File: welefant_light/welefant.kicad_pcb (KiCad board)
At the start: 2 copper layers, 80 x 90 mm, 97 parts, among them J1 Conn_01x02, J2 Conn_02x8_Odd_Even, J3 Conn_02x6_Odd_Even, Q1 AO3401A, Q2 AO3401A, Q3 AO3401A, SW1 DPDT, SW2 RESET, SW3 BOOT, U1 NCP167BMX330TBG, U2 Audio Jack PJ-324, U3 SD18OB261-060, U4 TP4056, U5 welefant, U7 ESP32-S3, U8 128MBit Flash, X1 40 MHz

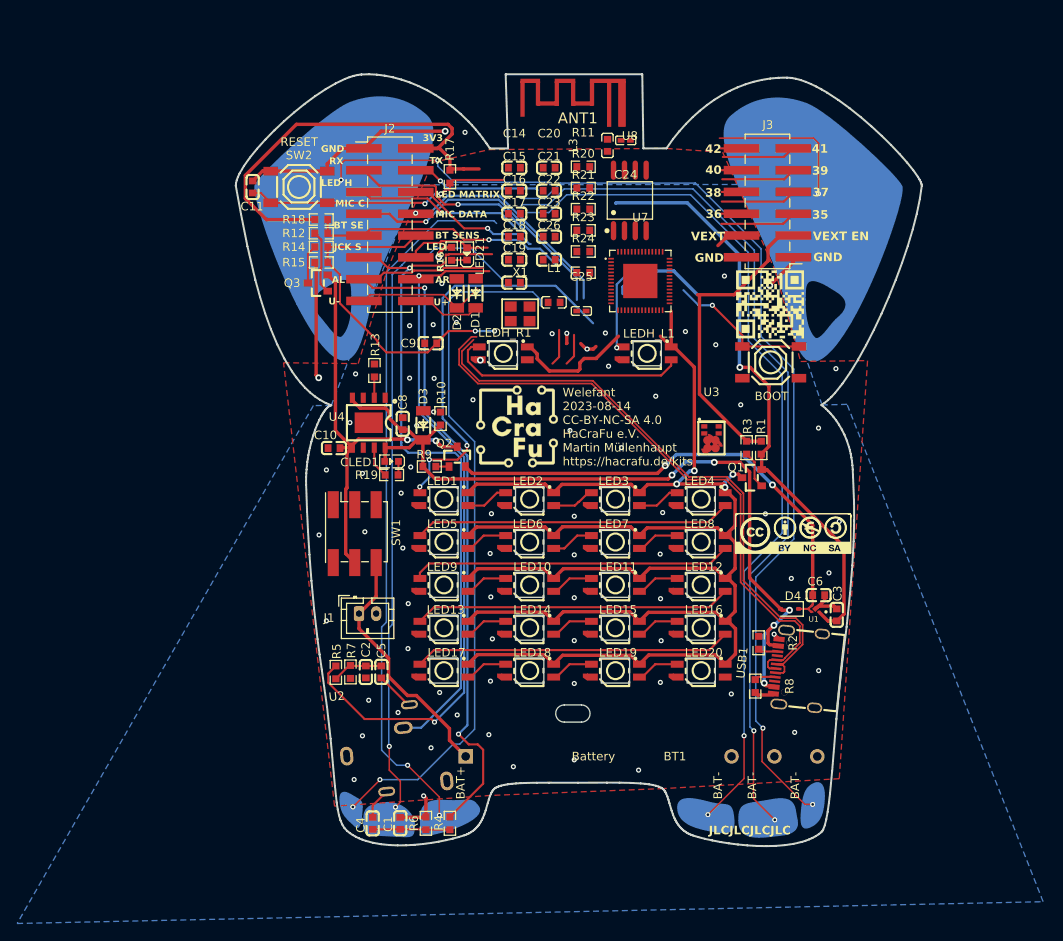
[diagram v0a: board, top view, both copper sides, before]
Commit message: weiter
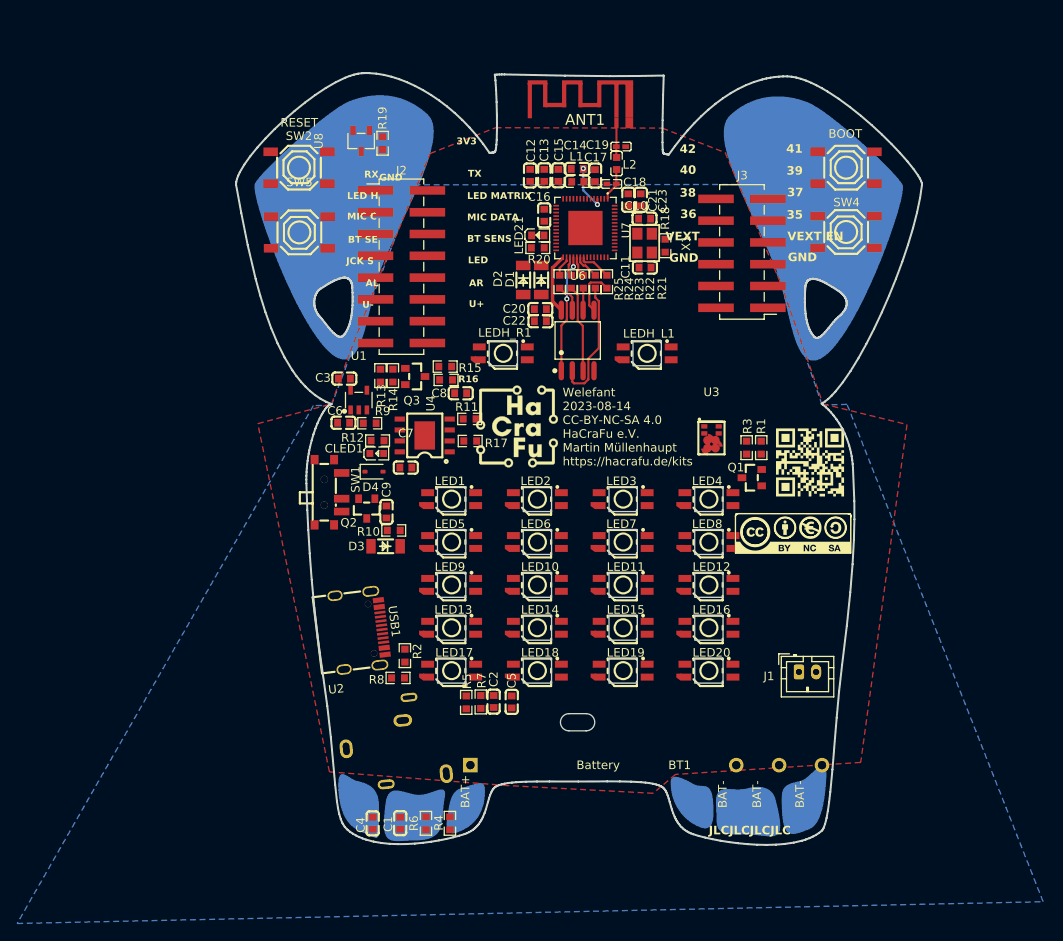
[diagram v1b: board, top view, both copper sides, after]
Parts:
- removed C24: 3p3, easyeda2kicad:C0402
- removed C25: 4p7, easyeda2kicad:C0402
- removed C26: 100n, easyeda2kicad:C0603
- removed L3: 2n2, easyeda2kicad:L0603
- added C12: 10u, easyeda2kicad:C0603, F.Cu at (66.3, 45.2)
- added C13: 1u, easyeda2kicad:C0603, F.Cu at (68.0, 45.2)
- added C7: 10u, easyeda2kicad:C0603, F.Cu at (51.9, 79.3)
- added L2: 2n2, easyeda2kicad:L0603, F.Cu at (76.4, 43.9)
- added R25: 0, easyeda2kicad:R0603, F.Cu at (69.8, 57.6)
- added SW4: GPIO33, easyeda2kicad:SW-SMD_4P-L5.1-W5.1-P3.70-LS6.5-TL-2, F.Cu at (103.2, 51.9)
- added SW5: GPIO33, easyeda2kicad:SW-SMD_4P-L5.1-W5.1-P3.70-LS6.5-TL-2, F.Cu at (39.5, 51.9)
- added U6: 128MBit Flash, easyeda2kicad:SOIC-8_L5.3-W5.3-P1.27-LS8.0-BL, F.Cu at (71.9, 64.5)
- C10: value 10u -> 15p
- C11: value 1u -> 15p
- C14: value 100n -> 1u
- C15: value 1u -> 100n
- C16, C17: value 15p -> 100n
- C18: value 100n -> 4p7; footprint easyeda2kicad:C0603 -> easyeda2kicad:C0402
- C19: value 100n -> 3p3; footprint easyeda2kicad:C0603 -> easyeda2kicad:C0402
- C23: value 10u -> 100n
- C3: value 1u -> 10u
- R10: value 10K -> 1K
- R11: value 0 -> 10K
- R12: value 1K -> 330
- R13: value 3K3 -> 10K; footprint easyeda2kicad:R0603_NEW -> easyeda2kicad:R0603
- R14: value 390K -> 1K
- R15: value 100K -> 390K
- R16: value 330 -> 100K
- R17: value 10K -> 3K3; footprint easyeda2kicad:R0603 -> easyeda2kicad:R0603_NEW
- R18: value 10K -> 0
- R19: value 330 -> 10K
- R20: value 0 -> 330
- R9: value 1K -> 100K
- SW1: value DPDT -> ON-OFF; footprint hacrafu:Switch_MSS22D18 -> easyeda2kicad:SW-SMD_MK-12C02-G025
- U1: value NCP167BMX330TBG -> RT9080-33GJ5; footprint hacrafu:XDFN-4 -> easyeda2kicad:TSOT-23-5_L2.9-W1.6-P0.95-LS2.8-BL
- U8: value 128MBit Flash -> Reset 2.8V; footprint easyeda2kicad:SOIC-8_L5.3-W5.3-P1.27-LS8.0-BL -> easyeda2kicad:SOT-23-3_L2.9-W1.6-P1.90-LS2.8-BR
- moved C3 63.7 mm to (44.7, 69.0), turned to 0 degrees
- moved C6 58.9 mm to (44.6, 74.1)
- moved U1 58.5 mm to (46.4, 71.5), turned to 0 degrees
- moved J1 51.7 mm to (97.7, 103.2)
- moved USB1 51.1 mm to (46.6, 98.3), turned to -83 degrees
- moved D4 51.0 mm to (48.1, 79.8), turned to 0 degrees
- moved C11 46.7 mm to (79.8, 56.0), turned to 0 degrees
- moved C10 45.0 mm to (79.7, 50.3)
- moved R8 41.7 mm to (51.0, 103.8), turned to 0 degrees
- moved R2 41.3 mm to (51.8, 101.2), turned to 90 degrees
- moved R18 40.2 mm to (82.1, 53.5), turned to -90 degrees
- moved R19 38.7 mm to (49.1, 41.5), turned to 90 degrees
- moved R11 32.2 mm to (59.3, 73.7), turned to 180 degrees
- moved U8 32.1 mm to (46.6, 41.2), turned to 90 degrees
- moved R17 30.9 mm to (59.4, 76.2), turned to 0 degrees
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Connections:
- BT1 pad 1: Net-(BT1-+) -> /VBAT
- C10 pad 1: GND -> /XTAL_N
- C10 pad 2: /VBAT -> GND
- C11 pad 1: /RESET -> GND
- C11 pad 2: GND -> Net-(X1-OSC2)
- C14 pad 1: GND -> /RESET
- C14 pad 2: /VDD_SPI -> GND
- C15 pad 1: /VDD_SPI -> GND
- C15 pad 2: GND -> /V33
- C16 pad 1: GND -> /V33
- C16 pad 2: Net-(X1-OSC2) -> GND
- C17 pad 1: /XTAL_N -> GND
- C17 pad 2: GND -> Net-(C17-Pad2)
- C18 pad 2: /V33 -> Net-(U7-LNA_IN)
- C19 pad 2: /V33 -> Net-(ANT1-PadFEED)
- C20 pad 2: Net-(C20-Pad2) -> /VDD_SPI
- C22 pad 1: GND -> /VDD_SPI
- C22 pad 2: /V33 -> GND
- C23 pad 1: /V33 -> GND
- C23 pad 2: GND -> /V33
- C6 pad 1: /VBUS -> GND
- C6 pad 2: GND -> /VBUS
- C8 pad 1: /V5 -> GND
- C8 pad 2: GND -> /BAT_SENS
- C9 pad 2: /BAT_SENS -> /VBAT
- D4 pad 1: /VBUS -> Net-(D4-K)
- J1 pad 1: Net-(BT1-+) -> /VBAT
- L1 pad 2: Net-(C20-Pad2) -> Net-(C17-Pad2)
- Q2 pad 2: /VBUS -> Net-(D4-K)
- R10 pad 1: GND -> Net-(Q2-G)
- R11 pad 1: Net-(U7-SPID) -> GND
- R11 pad 2: /SPID -> /V5
- R12 pad 1: Net-(Q3-G) -> Net-(CLED1-C)
- R12 pad 2: /BAT_SENS_EN -> Net-(U4-~{CHRG})
- R13 pad 1: Net-(U4-PROG) -> /V33
- R13 pad 2: GND -> /BAT_SENS_EN
- R14 pad 1: /BAT_SENS -> Net-(Q3-G)
- R14 pad 2: Net-(Q3-D) -> /BAT_SENS_EN
- R15 pad 2: GND -> Net-(Q3-D)
- R16 pad 1: GND -> /BAT_SENS
- R16 pad 2: Net-(LED21-C) -> GND
- R17 pad 1: /V33 -> Net-(U4-PROG)
- R17 pad 2: /RESET -> GND
- R18 pad 1: /V33 -> /XTAL_P
- R18 pad 2: /BAT_SENS_EN -> Net-(X1-OSC2)
- R19 pad 1: Net-(CLED1-C) -> /V33
- R19 pad 2: Net-(U4-~{CHRG}) -> /RESET
- R20 pad 1: Net-(U7-SPIQ) -> GND
- R20 pad 2: /SPIQ -> Net-(LED21-C)
- R21 pad 1: Net-(U7-SPICLK) -> Net-(U7-SPID)
- R21 pad 2: /SPICLK -> /SPID
- R22 pad 1: Net-(U7-SPIWP) -> Net-(U7-SPIQ)
- R22 pad 2: /SPIWP -> /SPIQ
- R23 pad 1: Net-(U7-SPIHD) -> Net-(U7-SPICLK)
- R23 pad 2: /SPIHD -> /SPICLK
- R24 pad 1: /XTAL_P -> Net-(U7-SPIWP)
- R24 pad 2: Net-(X1-OSC2) -> /SPIWP
- R9 pad 1: Net-(Q2-G) -> Net-(U1-EN)
- R9 pad 2: /V5 -> /VBUS
- SW1 pad 1: unconnected-(SW1-A1-Pad1) -> /VBUS
- SW1 pad 2: unconnected-(SW1-AB1-Pad2) -> Net-(D4-K)
- SW1 pad 4: Net-(BT1-+) -> unconnected-(SW1-Pad4)
- SW1 pad 5: /VBAT -> unconnected-(SW1-Pad5)
- SW2 pad 1: unconnected-(SW2-A-Pad1) -> /RESET
- U1 pad 1: /V33 -> /VBUS
- U1 pad 3: /VBUS -> Net-(U1-EN)
- U1 pad 4: /VBUS -> unconnected-(U1-NC-Pad4)
- U1 pad 5: GND -> /V33
- U7 pad 2: Net-(C20-Pad2) -> Net-(C17-Pad2)
- U7 pad 3: Net-(C20-Pad2) -> Net-(C17-Pad2)
- U7 pad 38: unconnected-(U7-GPIO33-Pad38) -> /GPIO33
- U7 pad 39: unconnected-(U7-GPIO34-Pad39) -> /GPIO34
- U8 pad 1: /SPICS0 -> /RESET
- U8 pad 2: /SPIQ -> GND
- U8 pad 3: /SPIWP -> /V33
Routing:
- net /VEXT: track 233.2 -> 0.00 mm, vias 4 -> 0
- net /V33: track 122.7 -> 0.00 mm, vias 1 -> 0
- net /TOUCH_T1: track 103.7 -> 0.00 mm, vias 2 -> 0
- net /TOUCH_T2: track 102.1 -> 0.00 mm, vias 2 -> 0
- net /TOUCH_T3: track 100.1 -> 0.00 mm, vias 2 -> 0
- net /V5: track 96.3 -> 0.00 mm, vias 5 -> 0
- net /AUDIO_PWM_L: track 88.0 -> 0.00 mm, vias 2 -> 0
- net /USB_DN: track 85.8 -> 0.00 mm
- net /TOUCH_T4: track 83.3 -> 0.00 mm, vias 2 -> 0
- net /TOUCH_T6: track 81.4 -> 0.00 mm, vias 2 -> 0
- net /JACK_SENS: track 80.7 -> 0.00 mm, vias 1 -> 0
- net /AUDIO_PWM_R: track 80.7 -> 0.00 mm, vias 2 -> 0
- net /TOUCH_T5: track 80.4 -> 0.00 mm, vias 2 -> 0
- net /USB_DP: track 79.0 -> 0.00 mm
- net /LED_MATRIX: track 63.9 -> 0.00 mm, vias 4 -> 0
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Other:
- outline, holes or cut-outs redrawn

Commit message: stand
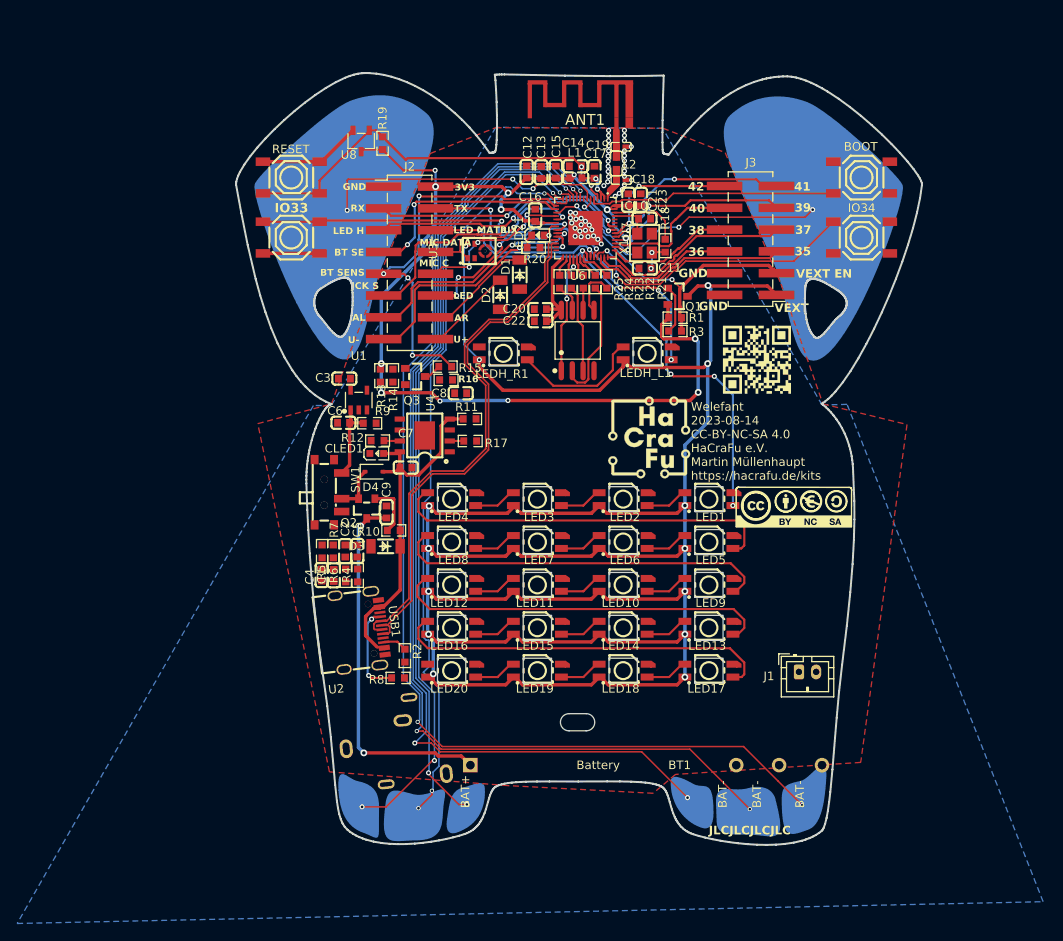
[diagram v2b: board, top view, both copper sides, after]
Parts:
- SW5: value GPIO33 -> IO34
- U3: footprint easyeda2kicad:MIC-SMD_SD18OB261-060 -> hacrafu:MIC-SMD_SD18OB261-060
- moved SW5 65.6 mm to (105.0, 52.5)
- moved SW4 64.7 mm to (38.5, 52.5)
- moved U3 34.8 mm to (60.3, 54.1), turned to 90 degrees
- moved R4 30.8 mm to (46.2, 91.9)
- moved R6 30.4 mm to (44.9, 91.9)
- moved LED1 30.0 mm to (87.2, 83.0), turned to 180 degrees
- moved LED12 30.0 mm to (57.2, 93.0), turned to 180 degrees
- moved LED13 30.0 mm to (87.2, 98.0), turned to 180 degrees
- moved LED16 30.0 mm to (57.2, 98.0), turned to 180 degrees
- moved LED17 30.0 mm to (87.2, 103.0), turned to 180 degrees
- moved LED20 30.0 mm to (57.2, 103.0), turned to 180 degrees
- moved LED4 30.0 mm to (57.2, 83.0), turned to 180 degrees
- moved LED5 30.0 mm to (87.2, 88.0), turned to 180 degrees
- moved LED8 30.0 mm to (57.2, 88.0), turned to 180 degrees
- moved LED9 30.0 mm to (87.2, 93.0), turned to 180 degrees
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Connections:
- J2 pad 10: /BAT_SENS -> /MIC_CLK
- J2 pad 14: /AUDIO_PWM_R -> /USB_DP
- J2 pad 15: /USB_DN -> /AUDIO_PWM_R
- J2 pad 16: /USB_DP -> /USB_DN
- J2 pad 4: /TX -> /LED_HEAD
- J2 pad 5: /LED_HEAD -> /TX
- J2 pad 7: /MIC_CLK -> /BAT_SENS_EN
- J2 pad 9: /BAT_SENS_EN -> /BAT_SENS
- J3 pad 1: GND -> /VEXT
- J3 pad 4: /VEXT -> GND
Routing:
- net /VEXT: track 0.00 -> 285.2 mm, vias 0 -> 14
- net /V33: track 0.00 -> 135.6 mm, vias 0 -> 13
- net /TOUCH_T1: track 0.00 -> 131.7 mm, vias 0 -> 3
- net /TOUCH_T2: track 0.00 -> 124.6 mm, vias 0 -> 3
- net /TOUCH_T3: track 0.00 -> 117.0 mm, vias 0 -> 3
- net /TOUCH_T6: track 0.00 -> 91.8 mm, vias 0 -> 3
- net /TOUCH_T4: track 0.00 -> 90.3 mm, vias 0 -> 3
- net /TOUCH_T5: track 0.00 -> 87.5 mm, vias 0 -> 3
- net /USB_DP: track 0.00 -> 74.3 mm
- net /USB_DN: track 0.00 -> 71.9 mm
- net /LED_MATRIX: track 0.00 -> 60.2 mm, vias 0 -> 5
- net /BAT_SENS: track 0.00 -> 45.6 mm, vias 0 -> 4
- net /D1_LED: track 0.00 -> 45.2 mm
- net /D4_LED: track 0.00 -> 44.7 mm
- net /D3_LED: track 0.00 -> 44.6 mm
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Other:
- board text added: "IO33"
- board text added: "IO34"

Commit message: stand
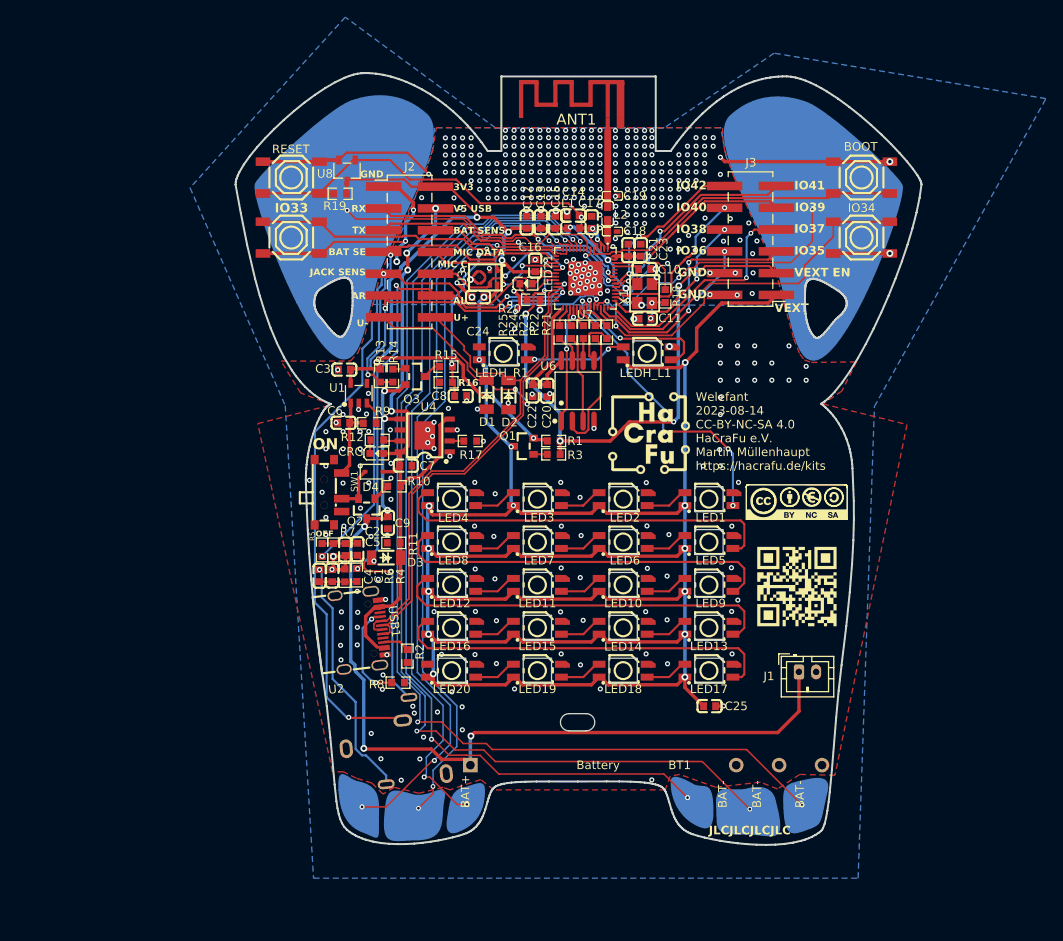
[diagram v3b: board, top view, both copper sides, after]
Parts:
- added C24: 100n, easyeda2kicad:C0603, F.Cu at (60.3, 59.5)
- added C25: 1u, easyeda2kicad:C0603, F.Cu at (87.3, 107.1)
- J2: value Conn_02x8_Odd_Even -> Conn_02x7_Odd_Even; footprint hacrafu:PinHeader_2x08_P2.54mm_Vertical_SMD_handsolder -> hacrafu:PinHeader_2x07_P2.54mm_Vertical_SMD_handsolder
- moved Q1 25.1 mm to (65.6, 76.8), turned to 0 degrees
- moved R1 20.2 mm to (69.1, 76.2)
- moved R3 20.2 mm to (69.1, 77.8)
- moved R11 16.9 mm to (50.5, 88.1), turned to 0 degrees
- moved D1 14.5 mm to (61.3, 70.8)
- moved D2 11.7 mm to (63.8, 70.9)
- moved C20 9.53 mm to (68.3, 70.3), turned to 90 degrees
- moved C22 8.15 mm to (66.7, 70.3), turned to -90 degrees
- moved R19 7.70 mm to (44.2, 47.4), turned to 180 degrees
- moved C18 6.11 mm to (76.0, 51.8)
- moved R20 6.08 mm to (66.8, 59.8)
- moved L2 5.94 mm to (75.4, 49.7)
- moved C10 5.87 mm to (79.7, 56.2)
- moved C16 5.87 mm to (67.0, 55.8)
- moved R21 5.87 mm to (75.3, 63.5)
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- renumbered CLED1 to CRG
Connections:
- J2 pad 11: /JACK_SENS -> /AUDIO_PWM_R
- J2 pad 12: /LED -> /AUDIO_PWM_L
- J2 pad 13: /AUDIO_PWM_L -> /USB_DP
- J2 pad 14: /USB_DP -> /USB_DN
- J2 pad 4: /LED_HEAD -> /V5
- J2 pad 6: /LED_MATRIX -> /BAT_SENS
- J2 pad 9: /BAT_SENS -> /JACK_SENS
- USB1 pad 1: (no net) -> unconnected-(USB1-SH-Pad1)
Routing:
- net GND: track 18.7 -> 101.2 mm, vias 46 -> 458
- net /VBAT: track 43.3 -> 110.6 mm, vias 2 -> 6
- net /JACK_SENS: track 28.3 -> 89.6 mm
- net /VEXT_EN: track 37.2 -> 70.0 mm, vias 2 -> 6
- net /V5: track 43.8 -> 76.0 mm, vias 0 -> 4
- net /AUDIO_PWM_L: track 27.1 -> 57.9 mm, vias 2 -> 4
- net Net-(C4-Pad2): track 0.00 -> 28.6 mm, vias 0 -> 1
- net /AUDIO_PWM_R: track 29.3 -> 57.8 mm, vias 2 -> 4
- net /LED_HEAD: track 43.1 -> 17.7 mm, vias 5 -> 2
- net /LED_MATRIX: track 60.2 -> 35.7 mm, vias 5 -> 4
- net /V33: track 135.6 -> 113.3 mm, vias 13 -> 9
- net Net-(C5-Pad2): track 0.00 -> 20.7 mm, vias 0 -> 1
- net /LED: track 20.2 -> 3.14 mm, vias 4 -> 0
- net /BAT_SENS_EN: track 25.2 -> 40.8 mm
- net /GPIO34: track 33.7 -> 45.6 mm
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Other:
- outline, holes or cut-outs redrawn
- board text added: "BAT SE"
- board text added: "BAT SENS"
- board text added: "IO35"
- board text added: "IO36"
- board text added: "IO37"
- board text added: "IO38"
- board text added: "IO39"
- board text added: "IO40"
- board text added: "IO41"
- board text added: "IO42"
- board text added: "JACK SENS"
- board text added: "OFF"
- board text added: "ON"
- board text added: "V5 USB"
- board text removed: "35"
- board text removed: "36"
- board text removed: "37"
- board text removed: "38"
- board text removed: "39"
- board text removed: "40"
- board text removed: "41"
- board text removed: "42"
- board text removed: "BT SE"
- board text removed: "BT SENS"
- board text removed: "JCK S"
- board text removed: "LED"
- board text removed: "LED H"
- board text removed: "LED MATRIX"
